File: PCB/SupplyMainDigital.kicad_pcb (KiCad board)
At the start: 2 copper layers, 102 parts, among them CON1 BARREL_JACK, P1 12V, P2 5V, P3 3V3, P4 GND, P5 PGM, P6 SERIAL, P7 I2C, P8 OUT, SW1 SW_PUSH, U1 TLC272, U10 LT3080, U11 LT3080, U2 MCP1501, U3 MCP1501, U4 TLV5616C, U5 dsPIC33EPXXXGP502, U6 LT3081, U7 MCP4131, U8 LM334Z, U9 MAX4080

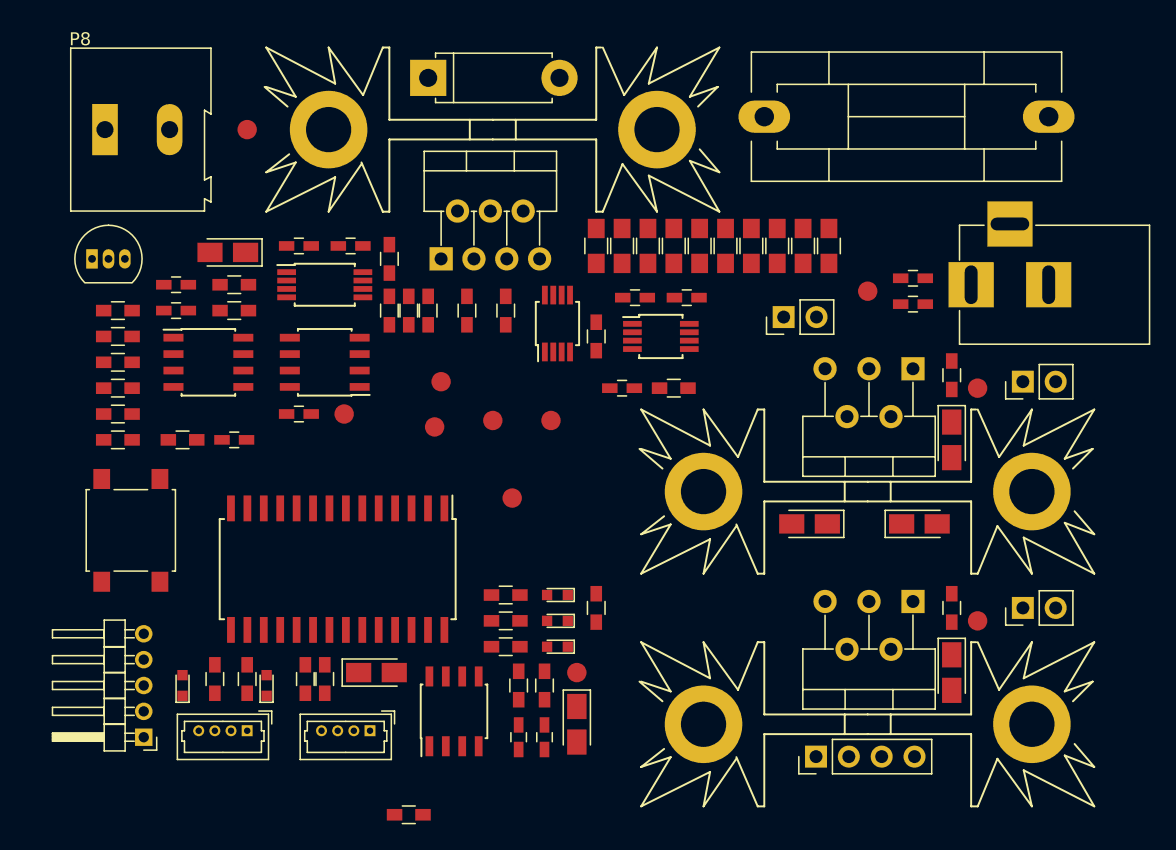
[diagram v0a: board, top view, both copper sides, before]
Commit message: Pcb layout V2 ready
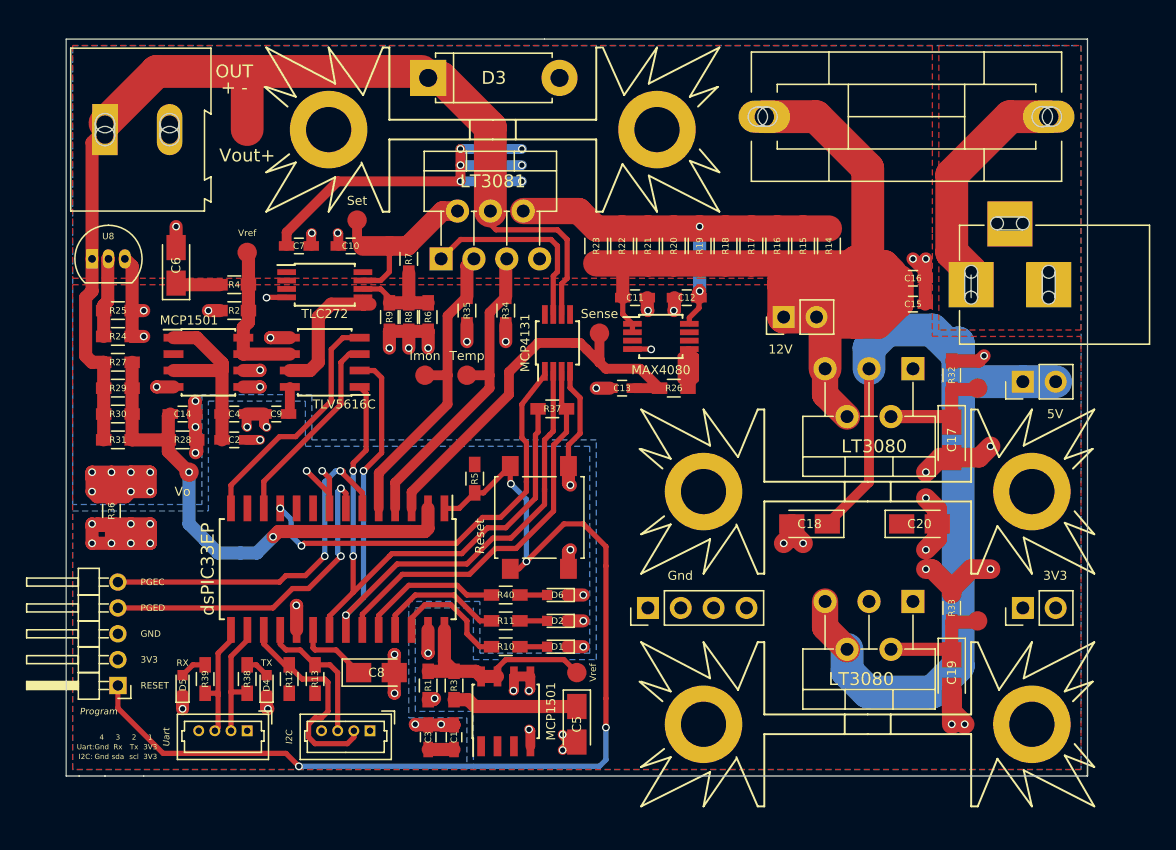
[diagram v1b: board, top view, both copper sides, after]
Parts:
- TP12: value Vo+ -> Vout+
- TP6: value Vout -> Vo
- TP7: value Temp -> Sense
- TP8: value Imon -> Temp
- TP9: value Sense -> Imon
- U5: value dsPIC33EPXXXGP502 -> dsPIC33EP
- moved R36 32.9 mm to (90.5, 81.5), turned to 270 degrees
- moved SW1 31.6 mm to (123.6, 82.0), turned to 270 degrees
- moved TP6 19.3 mm to (96.5, 78.5)
- moved P4 17.4 mm to (132.0, 89.0)
- moved TP2 14.6 mm to (101.0, 61.5)
- moved TP3 14.1 mm to (109.5, 59.0)
- moved R5 13.7 mm to (118.6, 79.0), turned to 90 degrees
- moved C2 11.0 mm to (100.0, 76.0)
- moved C4 11.0 mm to (100.0, 74.0)
- moved TP7 10.7 mm to (128.2, 67.8)
- moved TP9 10.4 mm to (114.8, 71.0)
- moved TP8 10.1 mm to (118.0, 71.0)
- moved C1 7.00 mm to (117.0, 99.0)
- moved C3 7.00 mm to (115.0, 99.0)
- moved R1 7.00 mm to (115.0, 95.0)
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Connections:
- TP7 pad 1: /TEMP -> /VSENSE
- TP8 pad 1: /IMON -> /TEMP
- TP9 pad 1: /VSENSE -> /IMON
- U5 pad 3: /TEMP -> /VSENSE
- U5 pad 4: /IMON -> /TEMP
- U5 pad 5: /VSENSE -> /IMON
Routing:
- net +12V: track 0.00 -> 121.8 mm, vias 0 -> 6
- net GNDA: track 0.00 -> 105.0 mm, vias 0 -> 50
- net /VO+: track 0.00 -> 83.9 mm
- net /RESET: track 0.00 -> 82.0 mm, vias 0 -> 4
- net +5V: track 0.00 -> 81.0 mm
- net GND: track 0.00 -> 66.8 mm, vias 0 -> 24
- net /SPI_SCK: track 0.00 -> 54.3 mm, vias 0 -> 2
- net /SPI_SDO: track 0.00 -> 45.1 mm, vias 0 -> 2
- net /VO_SENSE: track 0.00 -> 39.8 mm, vias 0 -> 2
- net /SPI_CS_MCP: track 0.00 -> 32.9 mm, vias 0 -> 2
- net /VSENSE: track 0.00 -> 32.4 mm
- net /3081_IN: track 0.00 -> 32.2 mm, vias 0 -> 2
- net /SPI_SDI: track 0.00 -> 30.7 mm
- net /PGM_PGEC: track 0.00 -> 27.9 mm, vias 0 -> 2
- net /PGM_PGED: track 0.00 -> 26.1 mm, vias 0 -> 2
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- added copper zone on F.Cu, net +12V
- added copper zone on F.Cu, net +3V3
- added copper zone on F.Cu, net /Power/Pin
- added copper zone on B.Cu, net GND
- added copper zone on B.Cu, net GNDA
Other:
- board outline added: 79 x 57 mm
- rule trace_min: 0.2 -> 0.1524
- rule via_min_drill: 0.3 -> 0.254
- rule via_min_size: 0.4 -> 0.381
- board text added: "+ -"
- board text added: "1"
- board text added: "12V"
- board text added: "2"
- board text added: "3"
- board text added: "3V3"
- board text added: "4"
- board text added: "5V"
- board text added: "GND"
- board text added: "Gnd"
- board text added: "I2C"
- board text added: "I2C:"
- board text added: "PGEC"
- board text added: "PGED"
- board text added: "Program"
- board text added: "RESET"
- board text added: "RX"
- board text added: "Reset"
- board text added: "Rx"
- board text added: "TX"
- board text added: "Tx"
- board text added: "Uart"
- board text added: "Uart:"
- board text added: "scl"
- board text added: "sda"
